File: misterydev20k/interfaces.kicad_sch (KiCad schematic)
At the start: 45 parts, among them J4 Micro_SD_Card_Det1, J5 HDMI_A, J6 Grove 1125S-4P, SW2 KEY1, SW3 KEY2

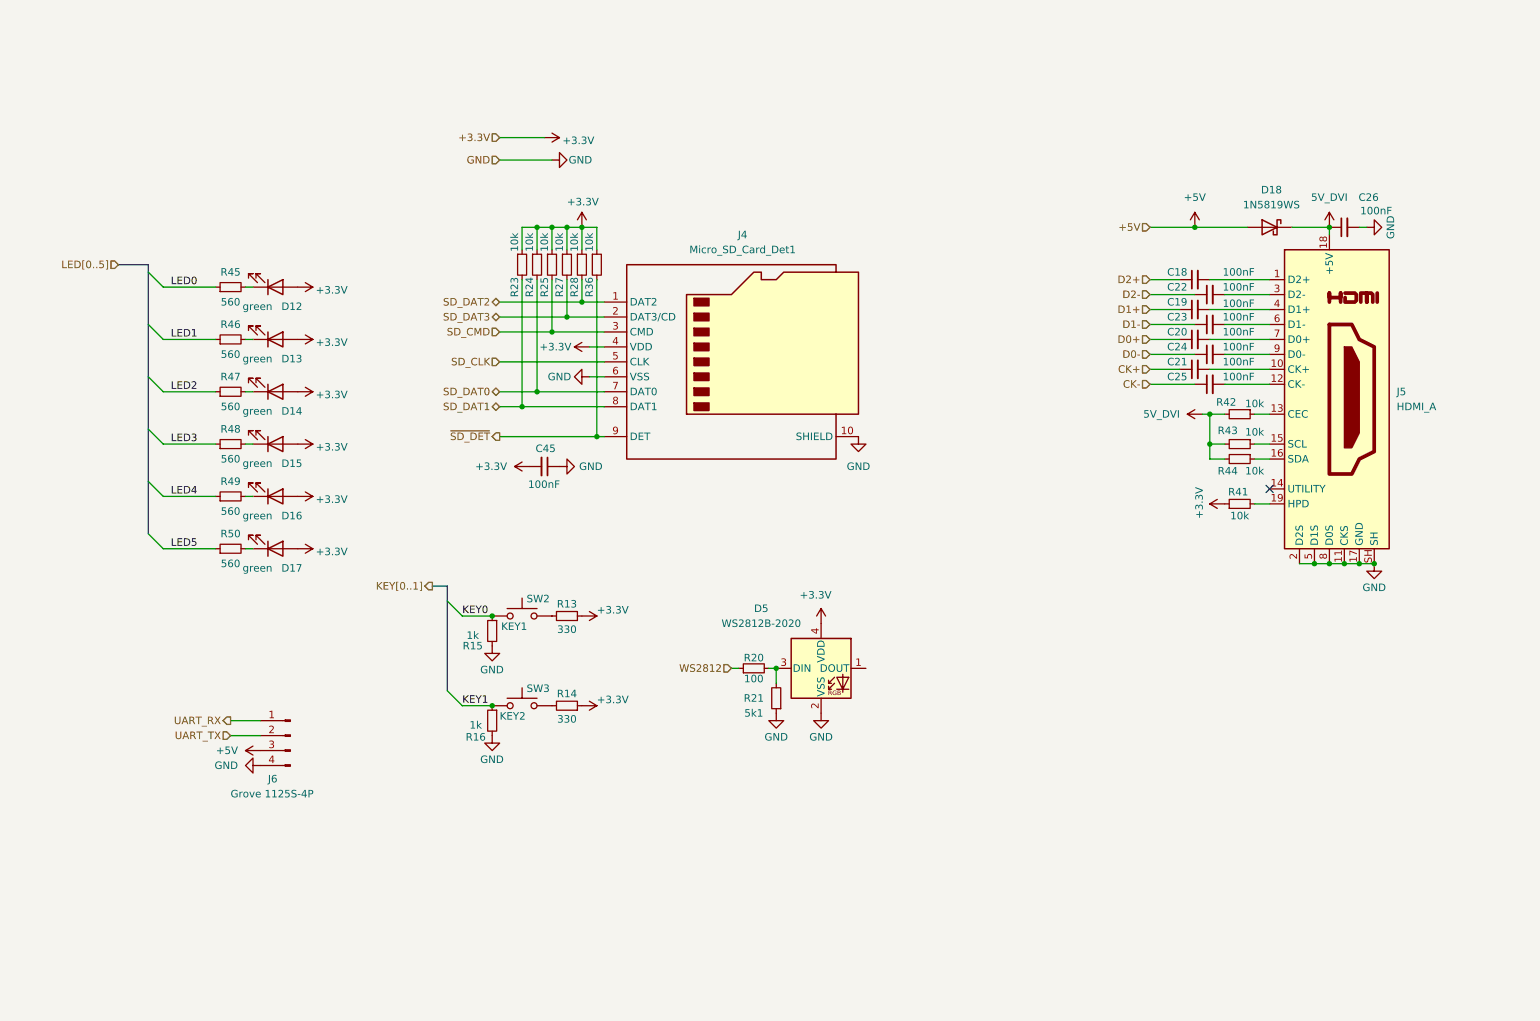
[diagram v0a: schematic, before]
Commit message: Update board
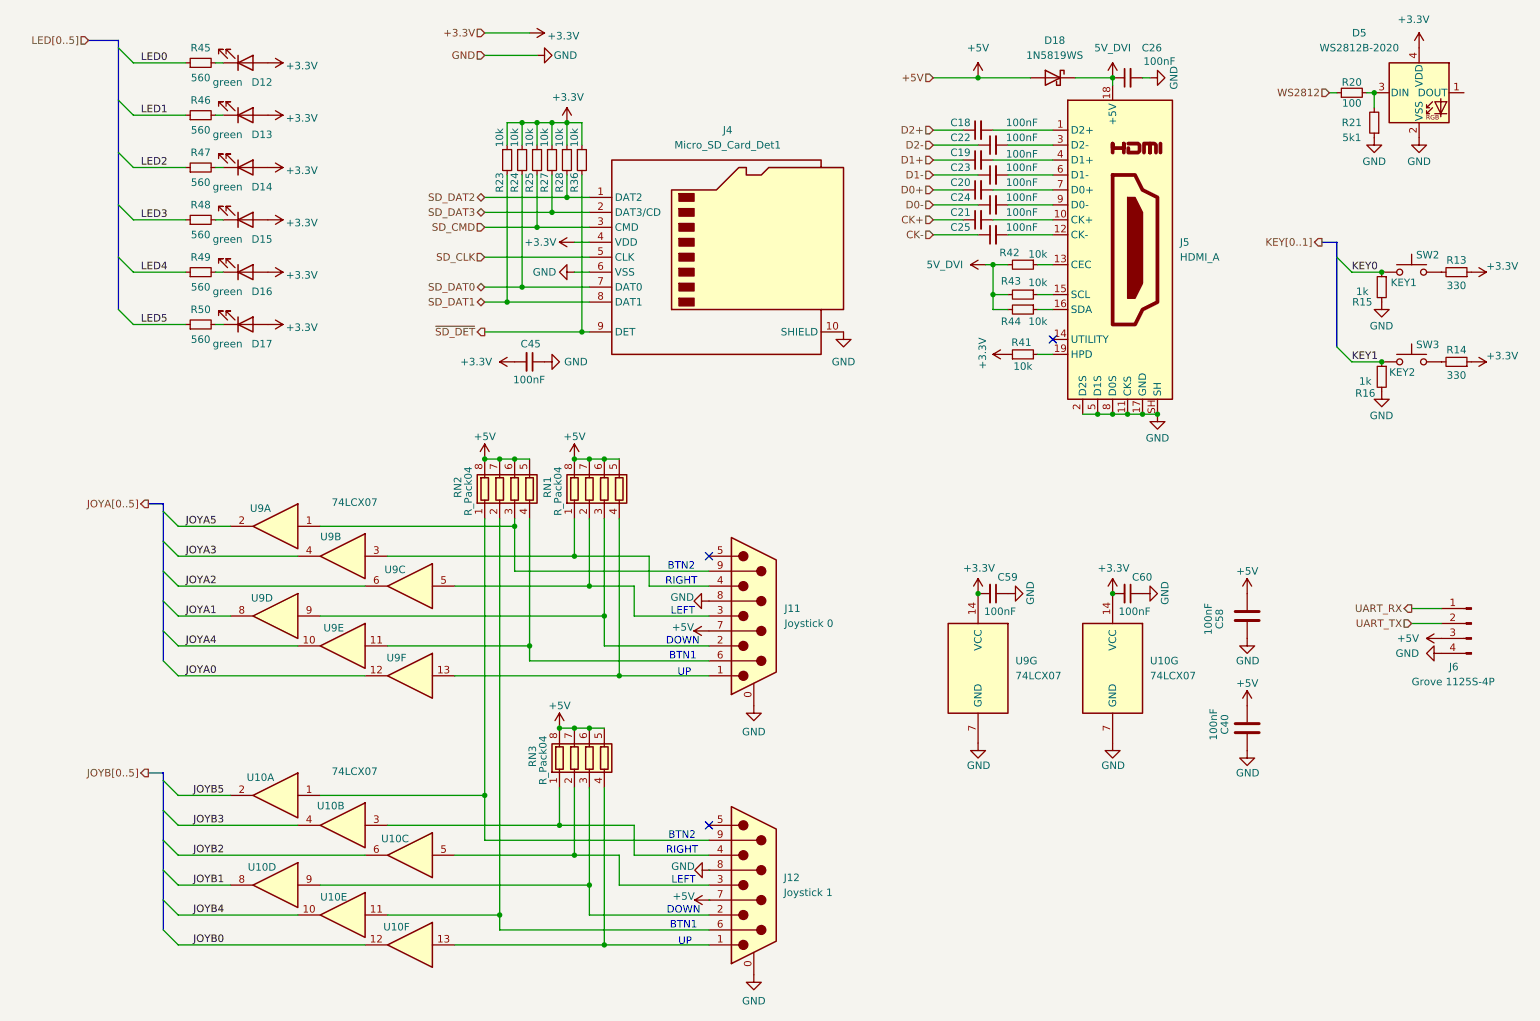
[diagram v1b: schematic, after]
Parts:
- added C40, C58: 100nF, Capacitor_SMD:C_0402_1005Metric, symbol Device:C
- added C59, C60: 100nF, Capacitor_SMD:C_0402_1005Metric, symbol Device:C_Small
- added J11: Joystick 0, Connector_Dsub:DSUB-9_Pins_Horizontal_P2.77x2.84mm_EdgePinOffset7.70mm_Housed_MountingHolesOffset9.12mm, symbol Connector:DE9_Plug_MountingHoles
- added J12: Joystick 1, Connector_Dsub:DSUB-9_Pins_Horizontal_P2.77x2.84mm_EdgePinOffset7.70mm_Housed_MountingHolesOffset9.12mm, symbol Connector:DE9_Plug_MountingHoles
- added RN1, RN2, RN3: R_Pack04, Resistor_SMD:R_Array_Concave_4x0603, symbol Device:R_Pack04
- added U10, U9: 74LCX07, Package_SO:TSSOP-14_4.4x5mm_P0.65mm, symbol 74xx:74LCX07
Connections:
- net +3.3V: now also C59.2, C60.2, U10.14 (VCC), U9.14 (VCC)
- net +5V: now also C40.2, C58.2, J11.7, J12.7, RN1.5 (R4.2), RN1.6 (R3.2), RN1.7 (R2.2), RN1.8 (R1.2), RN2.5 (R4.2), RN2.6 (R3.2), RN2.7 (R2.2), RN2.8 (R1.2), RN3.5 (R4.2), RN3.6 (R3.2), RN3.7 (R2.2), RN3.8 (R1.2)
- net GND: now also C40.1, C58.1, C59.1, C60.1, J11.0 (PAD), J11.8, J12.0 (PAD), J12.8, U10.7 (GND), U9.7 (GND)
- new net: J12.6, RN2.2 (R2.1), U10.11
- new net: J12.9, RN2.1 (R1.1), U10.1
- new net: J11.9, RN2.3 (R3.1), U9.1
- new net: J11.6, RN2.4 (R4.1), U9.11
- new net: J11.3, RN1.2 (R2.1), U9.5
- new net: J12.4, RN3.1 (R1.1), U10.3
- new net: J12.1, RN3.4 (R4.1), U10.13
- new net: J11.4, RN1.1 (R1.1), U9.3
- new net: J11.2, RN1.3 (R3.1), U9.9
- new net: J11.1, RN1.4 (R4.1), U9.13
- new net: J12.3, RN3.2 (R2.1), U10.5
- new net: J12.2, RN3.3 (R3.1), U10.9
- new net JOYA0: U9.12
- new net JOYA1: U9.8
- new net JOYA2: U9.6
- new net JOYA3: U9.4
- new net JOYA4: U9.10
- new net JOYA5: U9.2
- new net JOYB0: U10.12
- new net JOYB1: U10.8
- new net JOYB2: U10.6
- new net JOYB3: U10.4
- new net JOYB4: U10.10
- new net JOYB5: U10.2
- no-connect marks 1 -> 3
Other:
- note added: "BTN1"
- note added: "BTN2"
- note added: "DOWN"
- note added: "LEFT"
- note added: "RIGHT"
- note added: "UP"
- moved on the sheet: C18, C19, C20, C21, C22, C23, C24, C25, C26, C45, D12, D13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
